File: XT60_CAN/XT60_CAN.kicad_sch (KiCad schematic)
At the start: 28 parts, among them J1 XT60_IN, J10 mx3.0_2x2, J11 mx3.0_2x2, J12 mx3.0_2x2, J13 mx3.0_2x2, J14 mx3.0_2x2, J15 XT60_CH4, J16 XT60_CH5, J17 resistor, J18 resistor, J19 DC step down power, J2 XT60_CH1, J20 DC step down power, J3 mx3.0_2x2, J4 mx3.0_2x2, J5 mx3.0_2x2, J6 mx3.0_2x2, J7 mx3.0_2x2, J8 XT60_CH2, J9 XT60_CH3, U1 DCDC_StepDown_LM2596

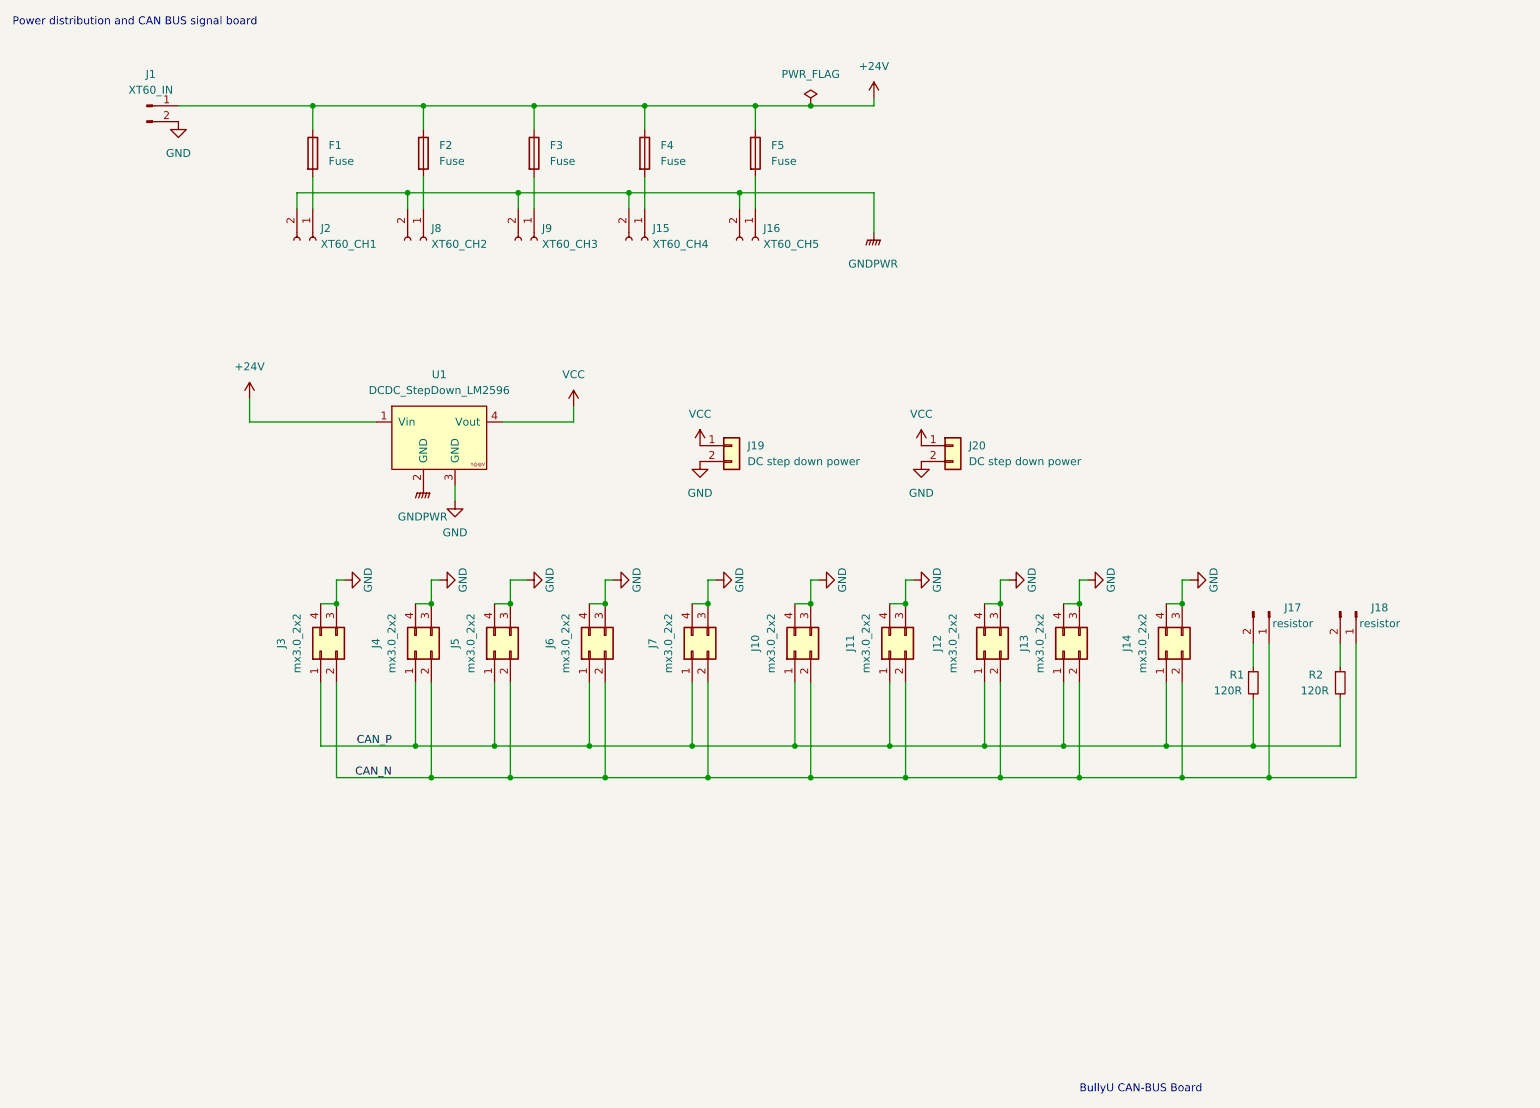
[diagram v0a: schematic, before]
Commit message: power_board
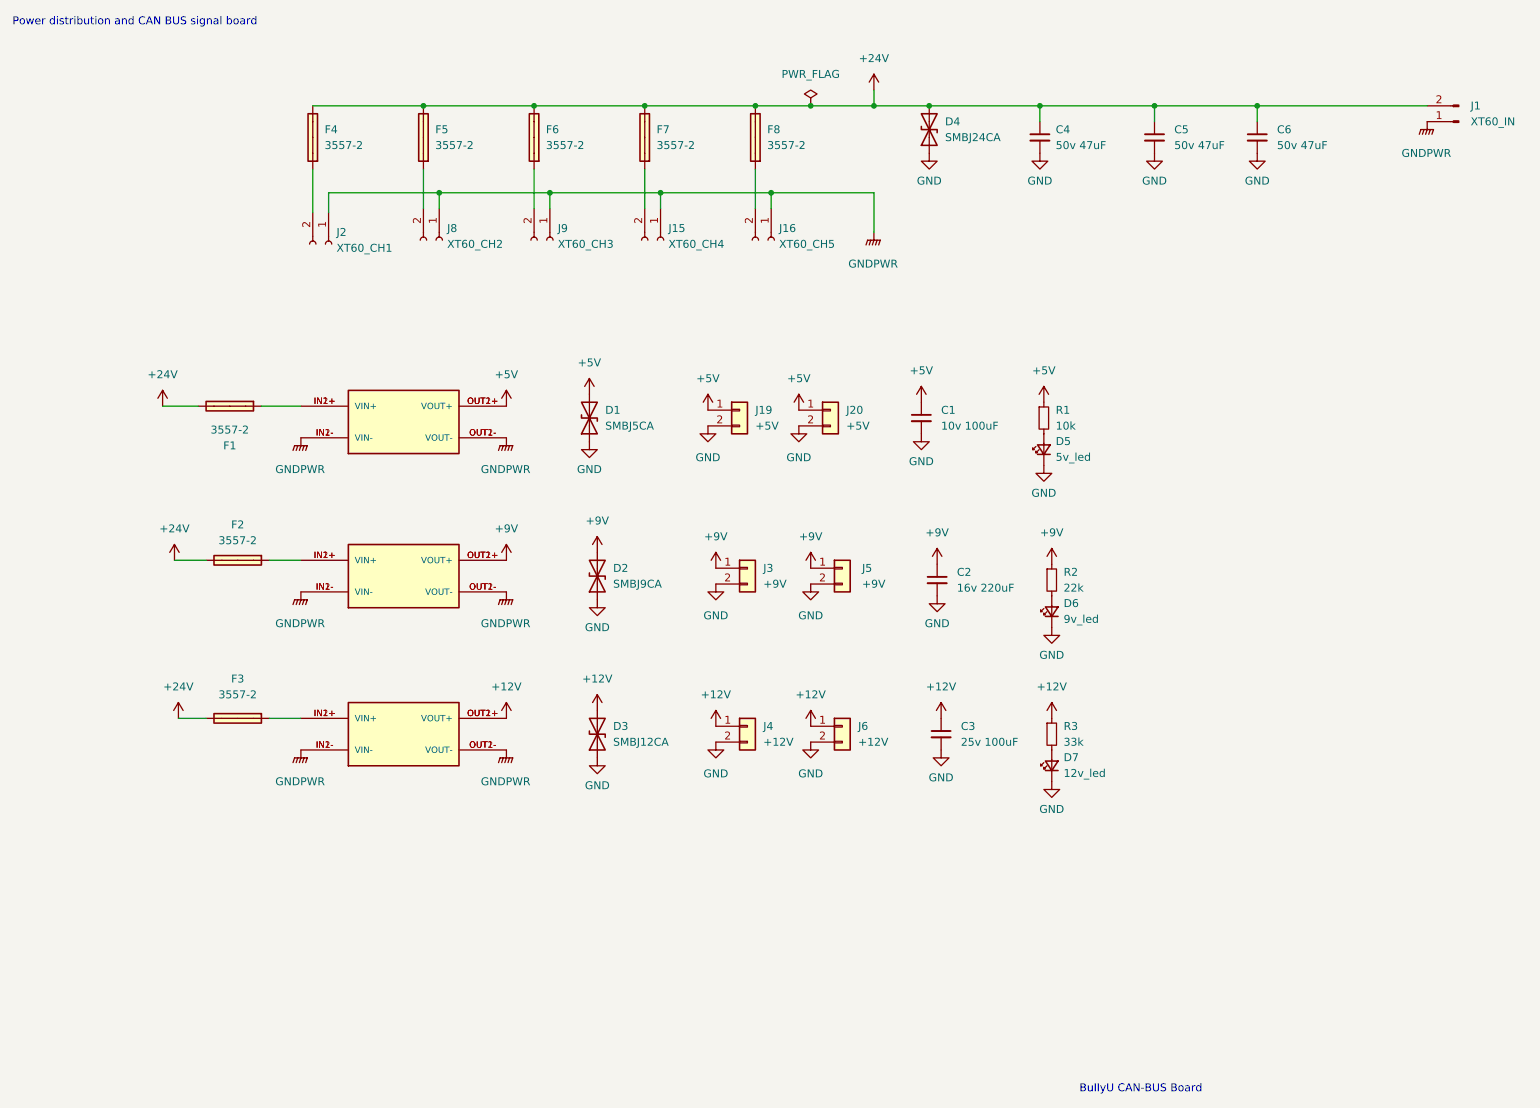
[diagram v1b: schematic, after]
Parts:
- removed F1, F2, F3, F4, F5: Fuse, Fuse_custom:Keystone_3557-2, symbol Device:Fuse
- removed J10, J11, J12, J13, J14, J3, J4, J5, J6, J7: mx3.0_2x2, Connector_Molex:Molex_Micro-Fit_3.0_43045-0412_2x02_P3.00mm_Vertical, symbol Connector_Generic:Conn_02x02_Counter_Clockwise
- removed J17, J18: resistor, Connector_PinHeader_2.54mm:PinHeader_1x02_P2.54mm_Vertical, symbol Connector:Conn_01x02_Male
- removed U1: DCDC_StepDown_LM2596, mid_DCDC2:YAAJ_DCDC_StepDown_LM2596, symbol yaaj_dcdc_stepdown_lm2596:YAAJ_DCDC_StepDown_LM2596
- added C1: 10v 100uF, Capacitor_SMD:C_Elec_5x5.4, symbol Device:C_Small
- added C2: 16v 220uF, Capacitor_SMD:C_Elec_6.3x7.7, symbol Device:C_Small
- added C3: 25v 100uF, Capacitor_SMD:C_Elec_6.3x7.7, symbol Device:C_Small
- added C4, C5, C6: 50v 47uF, Capacitor_SMD:C_Elec_6.3x7.7, symbol Device:C_Small
- added D1: SMBJ5CA, Diode_SMD:D_SMB, symbol Device:D_TVS
- added D2: SMBJ9CA, Diode_SMD:D_SMB, symbol Device:D_TVS
- added D3: SMBJ12CA, Diode_SMD:D_SMB, symbol Device:D_TVS
- added D4: SMBJ24CA, Diode_SMD:D_SMB, symbol Device:D_TVS
- added D5: 5v_led, LED_SMD:LED_0805_2012Metric_Pad1.15x1.40mm_HandSolder, symbol Device:LED_Small
- added D6: 9v_led, LED_SMD:LED_0805_2012Metric_Pad1.15x1.40mm_HandSolder, symbol Device:LED_Small
- added D7: 12v_led, LED_SMD:LED_0805_2012Metric_Pad1.15x1.40mm_HandSolder, symbol Device:LED_Small
- added F1, F2, F3, F4, F5, F6, F7, F8: 3557-2, PolyuRobotics:FUSE_3557-2, symbol PolyuRobotics:3557-2
- added J3, J5: +9V, Connector_Molex:Molex_Micro-Fit_3.0_43045-0212_2x01_P3.00mm_Vertical, symbol MP1584 Stepdown converter-cache:Connector_Generic_Conn_01x02
- added J4, J6: +12V, Connector_Molex:Molex_Micro-Fit_3.0_43045-0212_2x01_P3.00mm_Vertical, symbol MP1584 Stepdown converter-cache:Connector_Generic_Conn_01x02
- added R3: 33k, Resistor_SMD:R_0805_2012Metric_Pad1.20x1.40mm_HandSolder, symbol Device:R_Small
- added U1, U2, U3: MP1584, PolyuRobotics:DC-DC-mp1584_module, symbol PolyuRobotics:MP1584
- J19, J20: value DC step down power -> +5V
- R1: value 120R -> 10k
- R2: value 120R -> 22k
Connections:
- net VCC is gone; now on net +5V: J19.1 (Pin_1), J20.1 (Pin_1)
- net +24V: now also J1.2 (Pin_2), C4.1, C5.1, C6.1, D4.2 (A2), F1.2, F2.2, F3.2, F4.2, F5.2, F6.2, F7.2, F8.2; no longer J1.1 (Pin_1)
- net GND: now also C1.2, C2.2, C3.2, C4.2, C5.2, C6.2, D1.1 (A1), D2.1 (A1), D3.1 (A1), D4.1 (A1), D5.1 (K), D6.1 (K), D7.1 (K), J3.2 (Pin_2), J4.2 (Pin_2), J5.2 (Pin_2), J6.2 (Pin_2); no longer J1.2 (Pin_2)
- net GNDPWR: now also J1.1 (Pin_1), J15.1 (Pin_1), J16.1 (Pin_1), J2.1 (Pin_1), J8.1 (Pin_1), J9.1 (Pin_1), U1.IN1- (VIN-), U1.IN2- (VIN-), U1.OUT1- (VOUT-), U1.OUT2- (VOUT-), U2.IN1- (VIN-), U2.IN2- (VIN-), U2.OUT1- (VOUT-), U2.OUT2- (VOUT-), U3.IN1- (VIN-), U3.IN2- (VIN-), U3.OUT1- (VOUT-), U3.OUT2- (VOUT-); no longer J15.2 (Pin_2), J16.2 (Pin_2), J2.2 (Pin_2), J8.2 (Pin_2), J9.2 (Pin_2)
- net +5V: now reaches R1.1
- net +5V: now also C1.1, D1.2 (A2), U3.OUT1+ (VOUT+), U3.OUT2+ (VOUT+)
- net +9V: now reaches R2.1
- net +9V: now also C2.1, D2.2 (A2), J3.1 (Pin_1), J5.1 (Pin_1), U1.OUT1+ (VOUT+), U1.OUT2+ (VOUT+)
- net CAN_P: no longer names the net of R1.2
- net CAN_P: now also D5.2 (A); no longer R2.2
- new net: F2.1, U1.IN1+ (VIN+), U1.IN2+ (VIN+)
- new net: F8.1, J16.2 (Pin_2)
- new net: F3.1, U2.IN1+ (VIN+), U2.IN2+ (VIN+)
- new net: F6.1, J9.2 (Pin_2)
- new net: F4.1, J2.2 (Pin_2)
- new net: F1.1, U3.IN1+ (VIN+), U3.IN2+ (VIN+)
- new net: D6.2 (A), R2.2
- new net: F7.1, J15.2 (Pin_2)
- new net: F5.1, J8.2 (Pin_2)
- new net: D7.2 (A), R3.2
- new net +12V: C3.1, D3.2 (A2), J4.1 (Pin_1), J6.1 (Pin_1), R3.1, U2.OUT1+ (VOUT+), U2.OUT2+ (VOUT+)
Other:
- moved on the sheet: J1, J15, J16, J19, J2, J20, J8, J9
